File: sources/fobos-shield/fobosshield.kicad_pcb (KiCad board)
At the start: 2 copper layers, 83.8 x 63.5 mm, 155 parts, among them J1 Target, J10 ADCin, J11 PP1, J12 PP2, J13 Clock, J14 Trigger, J15 CSM5VCur, J16 Conn_01x01, J17 Barrel_Jack_Switch, J18 Conn_01x02, J19 Conn_01x02, J2 Glitch, J20 CSM3V3Cur, J21 GND, J22 GND, J3 Analog, J4 IOH, J5 SPI, J6 Analog2, J7 Power, J8 IOL, J9 SPI2, Q1 IRF7807Z, Q2 IRLML2502, Q3 BSS138L, U1 RB-0509D, U10 INA225, U11 INA225, U12 LD1117S33TR_SOT223, U2 REE-0505S, U3 LM317L_SO8, U4 LM337L_SO8, U5 LD59015, U6 LP3985IM5-3.0, U7 AD8331, U8 TPS7A7100_VQFN20, U9 AD9215

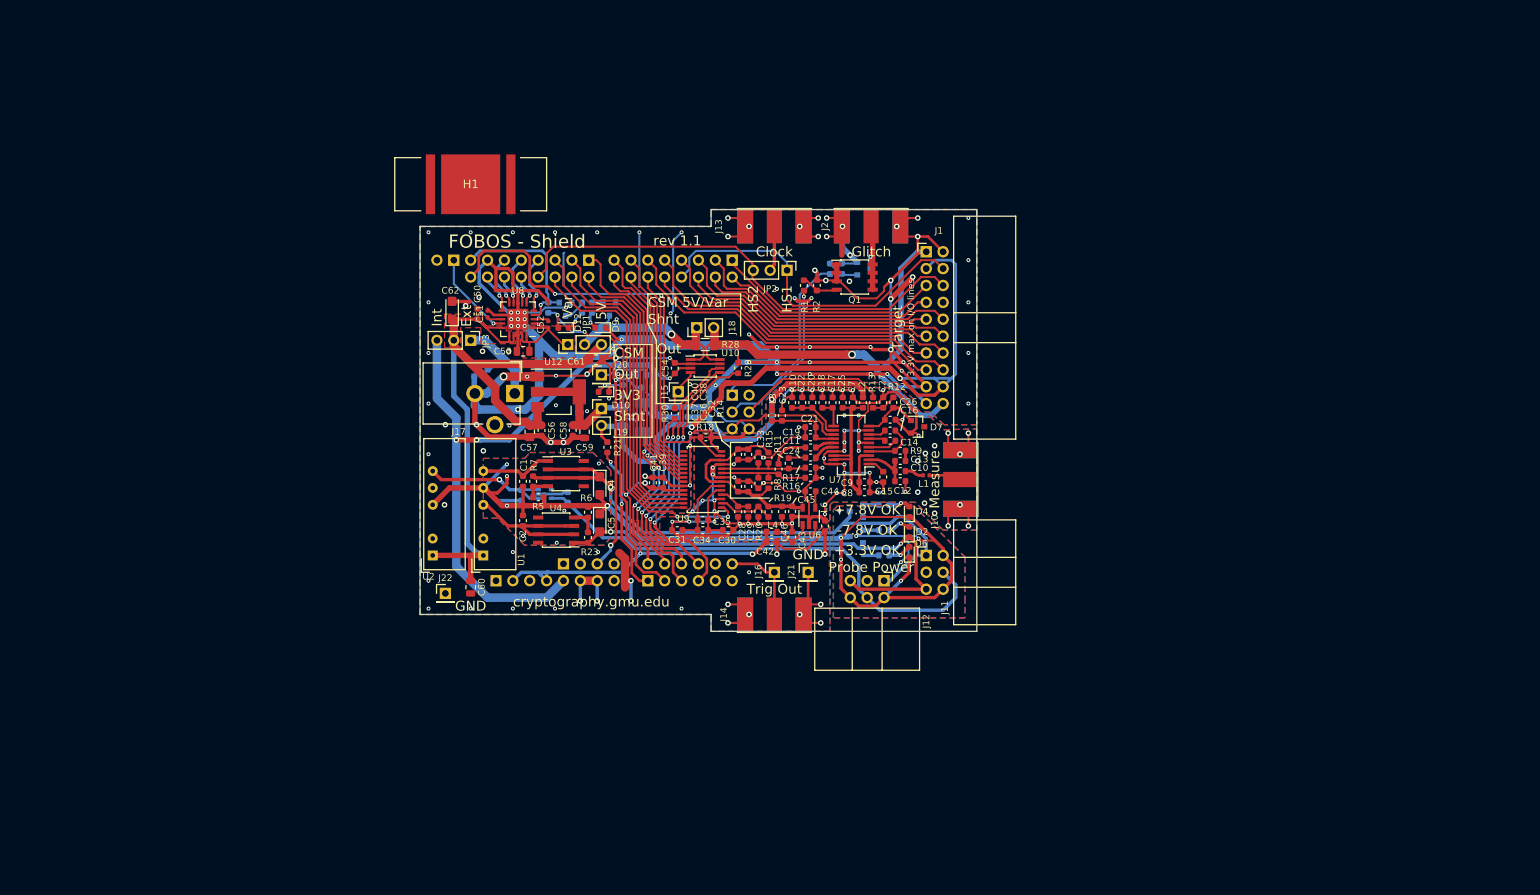
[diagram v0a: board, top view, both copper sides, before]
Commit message: trying new locations of components on shield
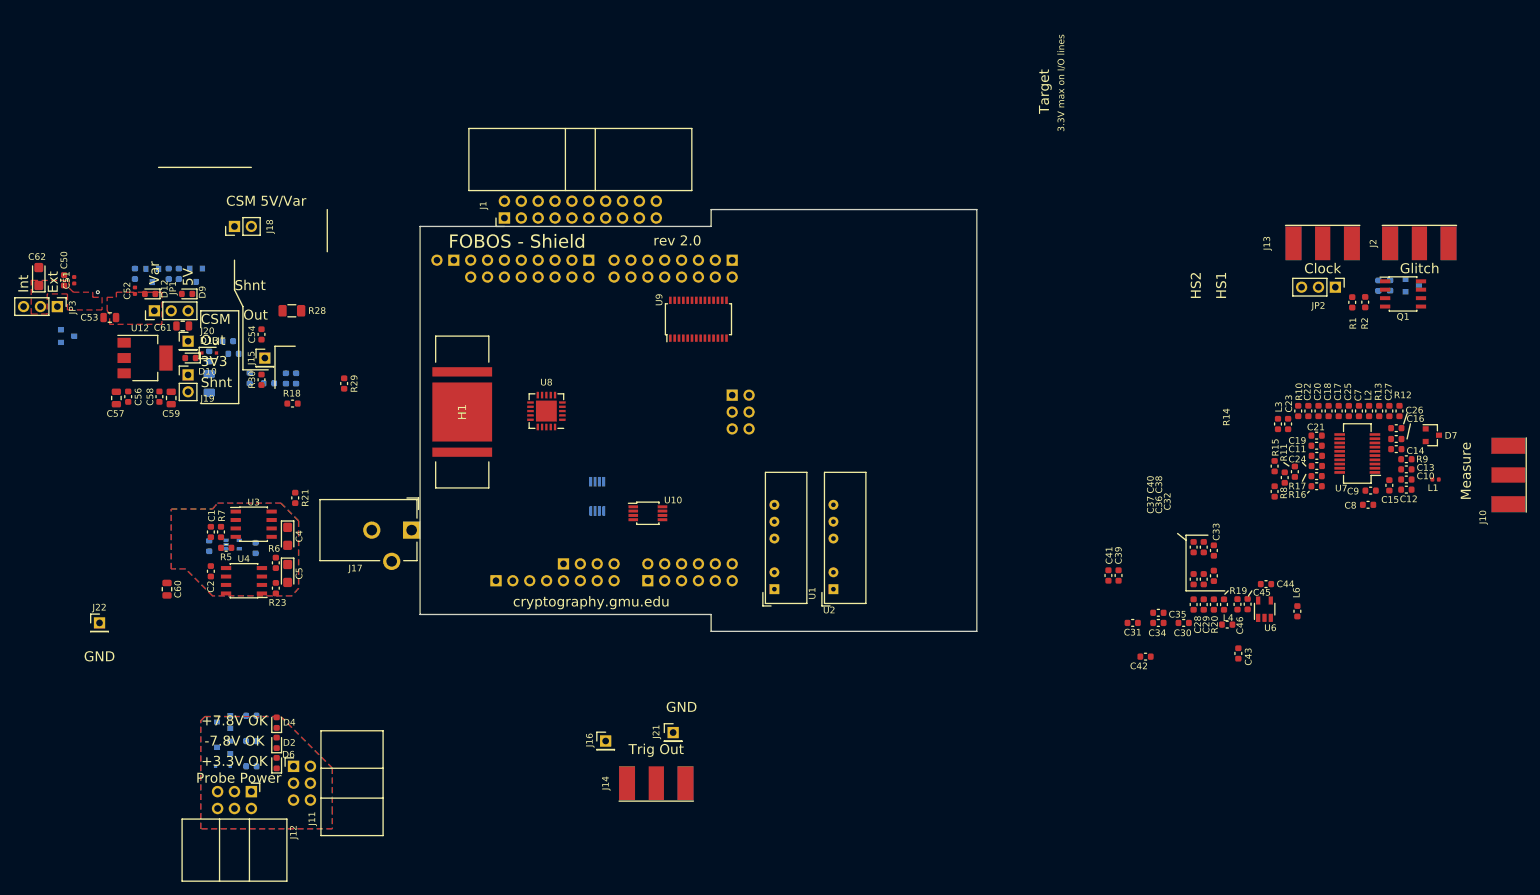
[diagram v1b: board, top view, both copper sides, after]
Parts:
- added D13: 1N4148, Diode_SMD:D_SOD-323F, F.Cu at (5.08, 44.5)
- R33: value 330R -> 100R
- moved D1 100.4 mm to (7.25, 100.0)
- moved D2 100.4 mm to (15.2, 103.1)
- moved D3 100.4 mm to (7.15, 106.7)
- moved D4 100.4 mm to (15.2, 100.1)
- moved D5 100.4 mm to (7.25, 103.8)
- moved D6 100.4 mm to (15.2, 106.2)
- moved J11 100.4 mm to (17.8, 106.7)
- moved J12 100.4 mm to (11.4, 110.5)
- moved R24 100.4 mm to (11.4, 99.1)
- moved R25 100.4 mm to (11.4, 102.9)
- moved R26 100.4 mm to (11.4, 106.7)
- moved Q1 82.6 mm to (184.8, 35.6)
- moved Q2 82.6 mm to (186.2, 34.3)
- moved R2 82.6 mm to (179.1, 36.8)
- moved J13 82.6 mm to (172.7, 27.9)
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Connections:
- J4 pad 1: ADC_D5 -> CW_SCK
- J4 pad 16: ADC_CLK -> CW_HS1
- J4 pad 2: ADC_D6 -> CW_TARG2
- J4 pad 3: ADC_D7 -> CW_MOSI
- J4 pad 4: ADC_D8 -> CW_TARG1
- J4 pad 5: ADC_D9 -> CW_MISO
- J4 pad 6: ADC_OR -> CW_RST
- J8 pad 1: CW_RST -> ADC_D1
- J8 pad 10: CW_TARG4 -> ADC_D7
- J8 pad 11: CW_PDID -> ADC_OR
- J8 pad 12: ADC_D0 -> ADC_D9
- J8 pad 13: ADC_D1 -> CW_PDID
- J8 pad 14: ADC_D2 -> CW_TARG4
- J8 pad 15: ADC_D3 -> CW_PDIC
- J8 pad 16: ADC_D4 -> CW_TARG3
- J8 pad 2: CW_MISO -> ADC_D0
- J8 pad 3: CW_TARG1 -> ADC_D3
- J8 pad 4: CW_MOSI -> ADC_D2
- J8 pad 5: CW_TARG2 -> ADC_D5
- J8 pad 6: CW_SCK -> ADC_D4
- J8 pad 7: CW_TARG3 -> ADC_D6
- J8 pad 8: CW_HS1 -> ADC_CLK
- J8 pad 9: CW_PDIC -> ADC_D8
- R33 pad 1: Net-(C58-Pad1) -> Net-(D13-Pad1)
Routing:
- net GND: track 553.6 -> 0.00 mm, vias 117 -> 1
- net GNDA: track 231.0 -> 0.00 mm, vias 66 -> 0
- net /Power/GNDP: track 181.3 -> 0.00 mm, vias 15 -> 0
- net IN: track 111.5 -> 0.00 mm
- net VCC5V0: track 110.2 -> 0.00 mm, vias 3 -> 0
- net CSM3V3: track 108.0 -> 0.00 mm, vias 2 -> 0
- net VCC3V3: track 103.1 -> 0.00 mm, vias 6 -> 0
- net /Power/+7V8P: track 88.7 -> 0.00 mm, vias 1 -> 0
- net /Power/3V3P: track 75.3 -> 0.00 mm
- net /Power/-7V8P: track 74.3 -> 0.00 mm, vias 2 -> 0
- net CSM5V: track 73.7 -> 0.00 mm, vias 1 -> 0
- net CW_HS2: track 72.5 -> 0.00 mm
- net ADC_CLK: track 69.5 -> 0.00 mm, vias 2 -> 0
- net ADC_OR: track 58.4 -> 0.00 mm, vias 2 -> 0
- net CW_HS1: track 52.4 -> 0.00 mm
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- removed copper zone on B.Cu, net GND
- removed copper zone on F.Cu, net GND
- removed copper zone on B.Cu, net GNDA
- removed copper zone on F.Cu, net GNDA
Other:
- board text added: "rev 2.0"
- board text removed: "rev 1.1"
